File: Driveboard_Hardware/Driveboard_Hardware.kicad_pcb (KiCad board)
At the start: 2 copper layers, 13 parts, among them U1 TM4C129E_Launchpad, U2 OKI, U3 MAX_3232

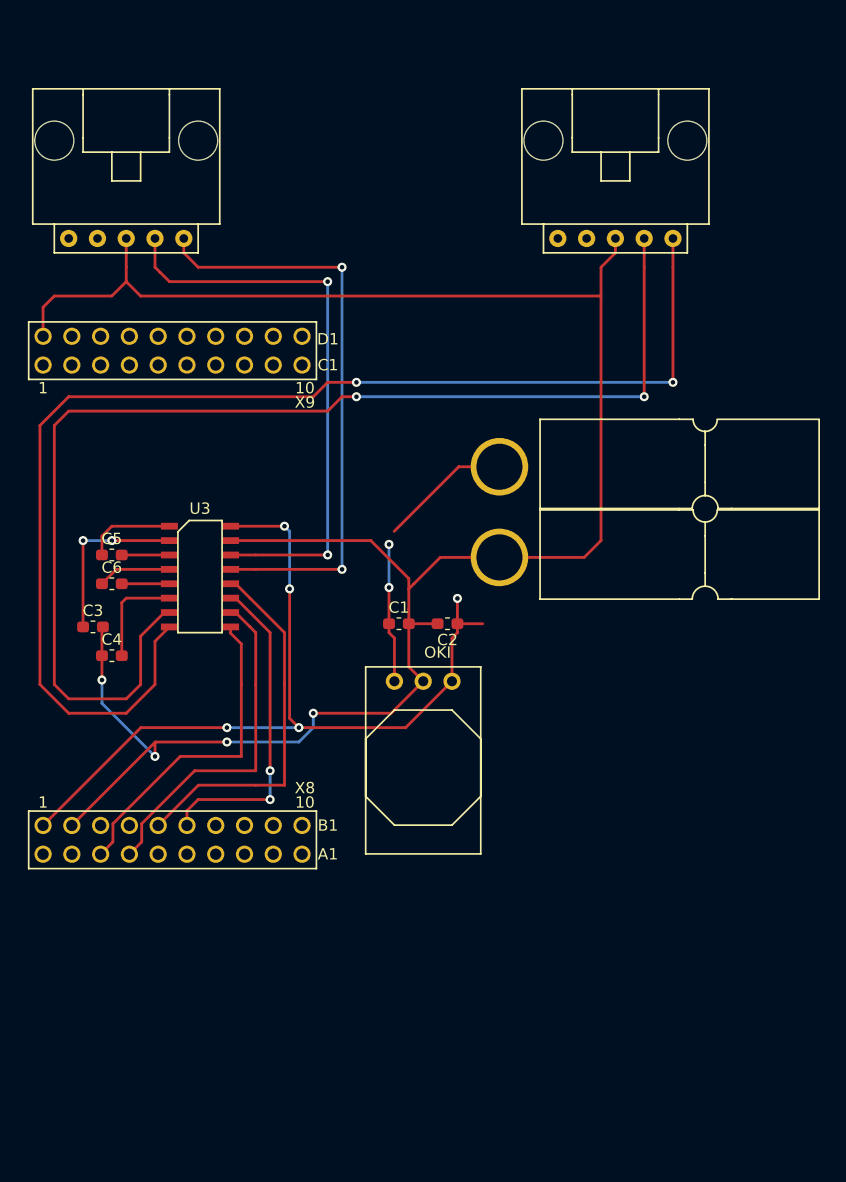
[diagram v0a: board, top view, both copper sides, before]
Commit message: Board Revised and Checked
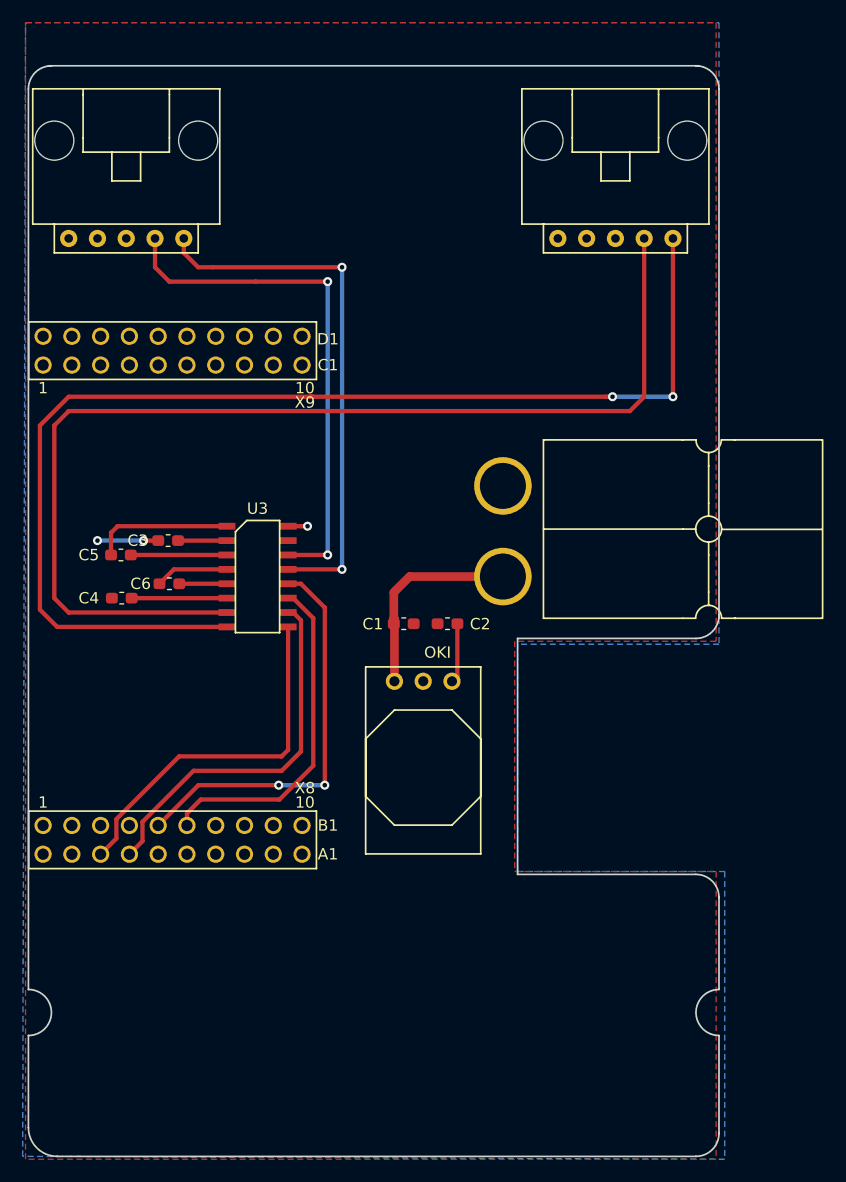
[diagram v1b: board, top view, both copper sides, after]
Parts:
- removed REF**: Anderson_1_Horisontal, MRDT_Connectors:Anderson_1_Horisontal
- C1, C2: value CP1_Small -> 10uF
- C3, C4, C5, C6: value CP1_Small -> .1uF
- Conn1: footprint MRDT_Connectors:Anderson_1_Horisontal -> MRDT_Connectors:Anderson_2_Horisontal_Side_by_Side
- Conn2: value Molex_SL_05 -> Motor1
- Conn3: value Molex_SL_05 -> Motor2
- moved C3 10.1 mm to (76.1, 104.1), turned to 180 degrees
- moved Conn1 6.19 mm to (109.2, 95.2)
- moved C4 5.15 mm to (72.0, 109.2)
- moved C6 5.08 mm to (76.2, 108.0)
- moved U3 5.08 mm to (84.0, 107.3)
- moved C5 0.80 mm to (71.9, 105.4)
- moved C1 0.43 mm to (96.9, 111.5)
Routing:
- net Earth: track 184.0 -> 5.36 mm, vias 4 -> 2
- net Net-(C2-Pad1): track 74.5 -> 6.99 mm, vias 5 -> 1
- net Net-(C1-Pad1): track 12.3 -> 41.0 mm, vias 2 -> 0
- net (no net): track 11.7 -> 0.00 mm
- net Net-(C3-Pad1): track 15.2 -> 4.32 mm, vias 2 -> 0
- net Net-(Conn3-Pad4): track 106.3 -> 98.5 mm, vias 2 -> 0
- net Net-(Conn3-Pad5): track 110.9 -> 104.6 mm
- net Net-(Conn2-Pad5): track 52.3 -> 47.2 mm
- net Net-(Conn2-Pad4): track 51.0 -> 45.9 mm
- net Net-(C5-Pad2): track 3.81 -> 8.48 mm
- net Net-(C5-Pad1): track 7.98 -> 12.4 mm
- net Net-(U1-PadPE2): track 32.6 -> 36.4 mm, vias 0 -> 2
- net Net-(U1-PadPC4): track 29.2 -> 32.7 mm
- net Net-(U1-PadPC5): track 30.3 -> 32.9 mm
- net Net-(U1-PadPE3): track 28.5 -> 29.9 mm, vias 2 -> 0
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- added copper zone on F.Cu, net Earth
- added copper zone on B.Cu, net Net-(C2-Pad1)
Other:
- board outline added: 61 x 96.3 mm
